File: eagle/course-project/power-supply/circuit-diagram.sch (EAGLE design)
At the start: 10 parts, among them IC1 7805T

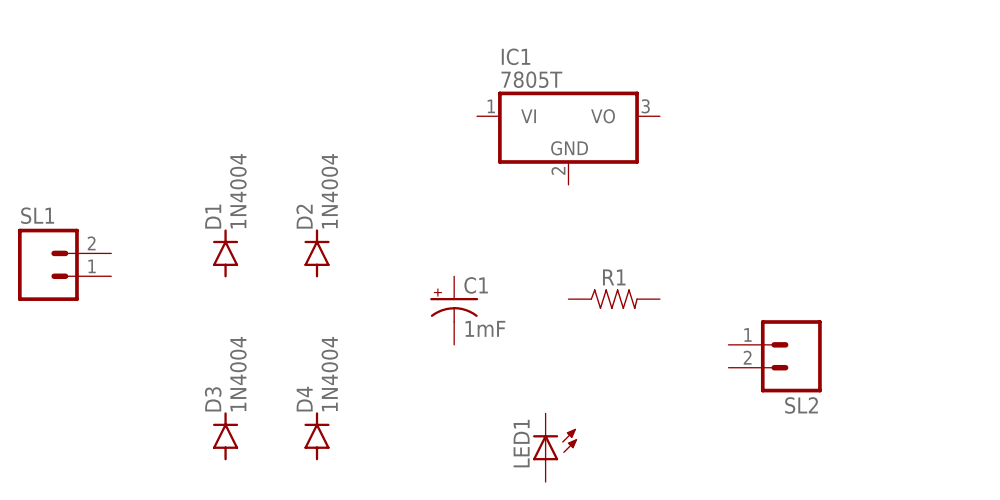
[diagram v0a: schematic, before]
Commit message: adding eagle files for practice
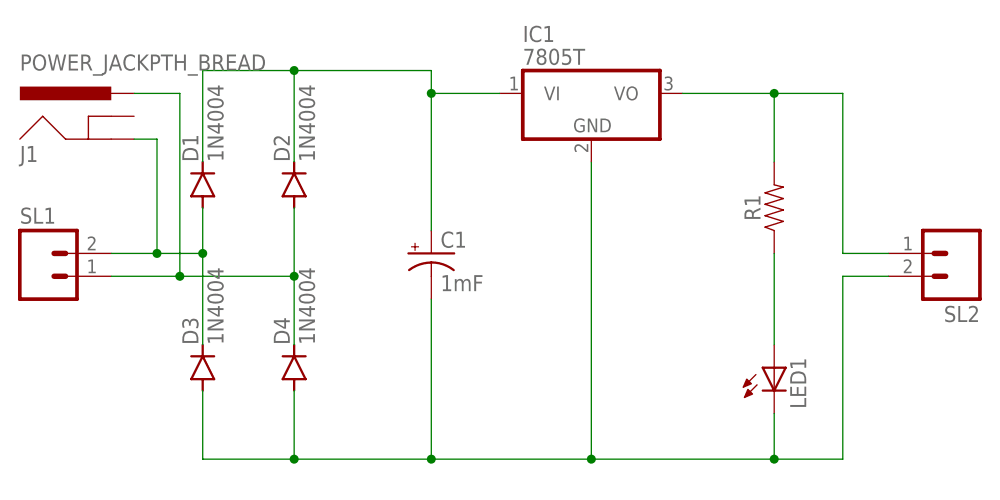
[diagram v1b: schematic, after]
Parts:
- added J1: POWER_JACKPTH_BREAD, SparkFun-Connectors:POWER_JACKPTH_BREAD
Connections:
- new net N$1: D1.A, D3.C, J1.GND, SL1.2
- new net N$2: C1.+, D1.C, D2.C, IC1.VI
- new net N$3: D2.A, D4.C, J1.PWR, SL1.1
- new net N$4: C1.-, D3.A, D4.A, IC1.GND, LED1.C, SL2.2
- new net N$5: IC1.VO, R1.2, SL2.1
- new net N$6: LED1.A, R1.1
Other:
- moved on the sheet: C1, D1, D2, D3, D4, IC1, LED1, R1, SL2
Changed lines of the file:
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@@
 <part name="LED1" library="adafruit" deviceset="LED" device="5MM"/>
 <part name="FRAME1" library="frames" library_urn="urn:adsk.eagle:library:229" deviceset="FRAME_A_L" device=""/>
+<part name="J1" library="SparkFun-Connectors" library_urn="urn:adsk.eagle:library:513" deviceset="POWER_JACK" device="PTH_BREAD" package3d_urn="urn:adsk.eagle:package:38228/1"/>
 </parts>
 <sheets>
@@
 <attribute name="NAME" x="35.56" y="74.422" size="1.778" layer="95"/>
 </instance>
-<instance part="SL2" gate="G$1" x="121.92" y="60.96" smashed="yes" rot="R180">
-<attribute name="VALUE" x="124.46" y="66.04" size="1.778" layer="96" rot="R180"/>
-<attribute name="NAME" x="124.46" y="55.118" size="1.778" layer="95" rot="R180"/>
+<instance part="SL2" gate="G$1" x="139.7" y="71.12" smashed="yes" rot="R180">
+<attribute name="VALUE" x="142.24" y="76.2" size="1.778" layer="96" rot="R180"/>
+<attribute name="NAME" x="142.24" y="65.278" size="1.778" layer="95" rot="R180"/>
 </instance>
-<instance part="D1" gate="1" x="58.42" y="71.12" smashed="yes" rot="R90">
-<attribute name="NAME" x="57.9374" y="73.66" size="1.778" layer="95" rot="R90"/>
-<attribute name="VALUE" x="60.7314" y="73.66" size="1.778" layer="96" rot="R90"/>
+<instance part="D1" gate="1" x="55.88" y="78.74" smashed="yes" rot="R90">
+<attribute name="NAME" x="55.3974" y="81.28" size="1.778" layer="95" rot="R90"/>
+<attribute name="VALUE" x="58.1914" y="81.28" size="1.778" layer="96" rot="R90"/>
 </instance>
-<instance part="D2" gate="1" x="68.58" y="71.12" smashed="yes" rot="R90">
-<attribute name="NAME" x="68.0974" y="73.66" size="1.778" layer="95" rot="R90"/>
-<attribute name="VALUE" x="70.8914" y="73.66" size="1.778" layer="96" rot="R90"/>
+<instance part="D2" gate="1" x="66.04" y="78.74" smashed="yes" rot="R90">
+<attribute name="NAME" x="65.5574" y="81.28" size="1.778" layer="95" rot="R90"/>
+<attribute name="VALUE" x="68.3514" y="81.28" size="1.778" layer="96" rot="R90"/>
 </instance>
-<instance part="D3" gate="1" x="58.42" y="50.8" smashed="yes" rot="R90">
-<attribute name="NAME" x="57.9374" y="53.34" size="1.778" layer="95" rot="R90"/>
-<attribute name="VALUE" x="60.7314" y="53.34" size="1.778" layer="96" rot="R90"/>
+<instance part="D3" gate="1" x="55.88" y="58.42" smashed="yes" rot="R90">
+<attribute name="NAME" x="55.3974" y="60.96" size="1.778" layer="95" rot="R90"/>
+<attribute name="VALUE" x="58.1914" y="60.96" size="1.778" layer="96" rot="R90"/>
 </instance>
-<instance part="D4" gate="1" x="68.58" y="50.8" smashed="yes" rot="R90">
-<attribute name="NAME" x="68.0974" y="53.34" size="1.778" layer="95" rot="R90"/>
-<attribute name="VALUE" x="70.8914" y="53.34" size="1.778" layer="96" rot="R90"/>
+<instance part="D4" gate="1" x="66.04" y="58.42" smashed="yes" rot="R90">
+<attribute name="NAME" x="65.5574" y="60.96" size="1.778" layer="95" rot="R90"/>
+<attribute name="VALUE" x="68.3514" y="60.96" size="1.778" layer="96" rot="R90"/>
 </instance>
-<instance part="C1" gate="G$1" x="83.82" y="66.04" smashed="yes">
-<attribute name="NAME" x="84.836" y="66.675" size="1.778" layer="95" font="vector"/>
-<attribute name="VALUE" x="84.836" y="61.849" size="1.778" layer="96" font="vector"/>
+<instance part="C1" gate="G$1" x="81.28" y="71.12" smashed="yes">
+<attribute name="NAME" x="82.296" y="71.755" size="1.778" layer="95" font="vector"/>
+<attribute name="VALUE" x="82.296" y="66.929" size="1.778" layer="96" font="vector"/>
 </instance>
-<instance part="IC1" gate="A1" x="96.52" y="86.36" smashed="yes">
-<attribute name="NAME" x="88.9" y="92.075" size="1.778" layer="95"/>
-<attribute name="VALUE" x="88.9" y="89.535" size="1.778" layer="96"/>
+<instance part="IC1" gate="A1" x="99.06" y="88.9" smashed="yes">
+<attribute name="NAME" x="91.44" y="94.615" size="1.778" layer="95"/>
+<attribute name="VALUE" x="91.44" y="92.075" size="1.778" layer="96"/>
 </instance>
-<instance part="R1" gate="G$1" x="101.6" y="66.04" smashed="yes">
-<attribute name="NAME" x="101.6" y="67.564" size="1.778" layer="95" font="vector" align="bottom-center"/>
-<attribute name="VALUE" x="101.6" y="64.516" size="1.778" layer="96" font="vector" align="top-center"/>
+<instance part="R1" gate="G$1" x="119.38" y="76.2" smashed="yes" rot="R90">
+<attribute name="NAME" x="117.856" y="76.2" size="1.778" layer="95" font="vector" rot="R90" align="bottom-center"/>
+<attribute name="VALUE" x="120.904" y="76.2" size="1.778" layer="96" font="vector" rot="R90" align="top-center"/>
 </instance>
-<instance part="LED1" gate="G$1" x="93.98" y="48.26" smashed="yes" rot="R180">
-<attribute name="NAME" x="90.424" y="52.832" size="1.778" layer="95" rot="R270"/>
-<attribute name="VALUE" x="88.265" y="52.832" size="1.778" layer="96" rot="R270"/>
+<instance part="LED1" gate="G$1" x="119.38" y="58.42" smashed="yes">
+<attribute name="NAME" x="122.936" y="53.848" size="1.778" layer="95" rot="R90"/>
+<attribute name="VALUE" x="125.095" y="53.848" size="1.778" layer="96" rot="R90"/>
 </instance>
 <instance part="FRAME1" gate="G$1" x="27.94" y="35.56" smashed="yes"/>
@@
 <attribute name="DRAWING_NAME" x="218.44" y="54.61" size="2.54" layer="94"/>
 </instance>
+<instance part="J1" gate="G$1" x="45.72" y="81.28" smashed="yes">
+<attribute name="VALUE" x="35.56" y="91.44" size="1.778" layer="96" font="vector"/>
+<attribute name="NAME" x="35.56" y="81.28" size="1.778" layer="95" font="vector"/>
+</instance>
 </instances>
 <busses>
 </busses>
 <nets>
+<net name="N$1" class="0">
+<segment>
+<pinref part="SL1" gate="G$1" pin="2"/>
+<wire x1="45.72" y1="71.12" x2="50.8" y2="71.12" width="0.1524" layer="91"/>
+<pinref part="D1" gate="1" pin="A"/>
+<wire x1="50.8" y1="71.12" x2="55.88" y2="71.12" width="0.1524" layer="91"/>
+<wire x1="55.88" y1="71.12" x2="55.88" y2="76.2" width="0.1524" layer="91"/>
+<pinref part="D3" gate="1" pin="C"/>
+<wire x1="55.88" y1="60.96" x2="55.88" y2="71.12" width="0.1524" layer="91"/>
+<junction x="55.88" y="71.12"/>
+<pinref part="J1" gate="G$1" pin="GND"/>
+<wire x1="48.26" y1="83.82" x2="50.8" y2="83.82" width="0.1524" layer="91"/>
+<wire x1="50.8" y1="83.82" x2="50.8" y2="71.12" width="0.1524" layer="91"/>
+<junction x="50.8" y="71.12"/>
+</segment>
+</net>
+<net name="N$2" class="0">
+<segment>
+<pinref part="D1" gate="1" pin="C"/>
+<wire x1="55.88" y1="81.28" x2="55.88" y2="91.44" width="0.1524" layer="91"/>
+<wire x1="55.88" y1="91.44" x2="66.04" y2="91.44" width="0.1524" layer="91"/>
+<pinref part="D2" gate="1" pin="C"/>
+<wire x1="66.04" y1="91.44" x2="66.04" y2="81.28" width="0.1524" layer="91"/>
+<wire x1="66.04" y1="91.44" x2="81.28" y2="91.44" width="0.1524" layer="91"/>
+<junction x="66.04" y="91.44"/>
+<pinref part="C1" gate="G$1" pin="+"/>
+<wire x1="81.28" y1="91.44" x2="81.28" y2="88.9" width="0.1524" layer="91"/>
+<pinref part="IC1" gate="A1" pin="VI"/>
+<wire x1="81.28" y1="88.9" x2="81.28" y2="73.66" width="0.1524" layer="91"/>
+<wire x1="88.9" y1="88.9" x2="81.28" y2="88.9" width="0.1524" layer="91"/>
+<junction x="81.28" y="88.9"/>
+</segment>
+</net>
+<net name="N$3" class="0">
+<segment>
+<pinref part="D2" gate="1" pin="A"/>
+<pinref part="D4" gate="1" pin="C"/>
+<wire x1="66.04" y1="76.2" x2="66.04" y2="68.58" width="0.1524" layer="91"/>
+<pinref part="SL1" gate="G$1" pin="1"/>
+<wire x1="66.04" y1="68.58" x2="66.04" y2="60.96" width="0.1524" layer="91"/>
+<junction x="66.04" y="68.58"/>
+<wire x1="45.72" y1="68.58" x2="53.34" y2="68.58" width="0.1524" layer="91"/>
+<pinref part="J1" gate="G$1" pin="PWR"/>
+<wire x1="53.34" y1="68.58" x2="66.04" y2="68.58" width="0.1524" layer="91"/>
+<wire x1="48.26" y1="88.9" x2="53.34" y2="88.9" width="0.1524" layer="91"/>
+<wire x1="53.34" y1="88.9" x2="53.34" y2="68.58" width="0.1524" layer="91"/>
+<junction x="53.34" y="68.58"/>
+</segment>
+</net>
+<net name="N$4" class="0">
+<segment>
+<pinref part="D3" gate="1" pin="A"/>
+<wire x1="55.88" y1="55.88" x2="55.88" y2="48.26" width="0.1524" layer="91"/>
+<wire x1="55.88" y1="48.26" x2="66.04" y2="48.26" width="0.1524" layer="91"/>
+<pinref part="D4" gate="1" pin="A"/>
+<wire x1="66.04" y1="48.26" x2="66.04" y2="55.88" width="0.1524" layer="91"/>
+<pinref part="C1" gate="G$1" pin="-"/>
+<wire x1="81.28" y1="66.04" x2="81.28" y2="48.26" width="0.1524" layer="91"/>
+<wire x1="81.28" y1="48.26" x2="66.04" y2="48.26" width="0.1524" layer="91"/>
+<junction x="66.04" y="48.26"/>
+<pinref part="IC1" gate="A1" pin="GND"/>
+<wire x1="99.06" y1="81.28" x2="99.06" y2="48.26" width="0.1524" layer="91"/>
+<wire x1="99.06" y1="48.26" x2="81.28" y2="48.26" width="0.1524" layer="91"/>
+<junction x="81.28" y="48.26"/>
+<wire x1="99.06" y1="48.26" x2="119.38" y2="48.26" width="0.1524" layer="91"/>
+<junction x="99.06" y="48.26"/>
+<pinref part="LED1" gate="G$1" pin="C"/>
+<wire x1="119.38" y1="48.26" x2="119.38" y2="53.34" width="0.1524" layer="91"/>
+<wire x1="127" y1="68.58" x2="127" y2="48.26" width="0.1524" layer="91"/>
+<wire x1="127" y1="48.26" x2="119.38" y2="48.26" width="0.1524" layer="91"/>
+<junction x="119.38" y="48.26"/>
+<pinref part="SL2" gate="G$1" pin="2"/>
+<wire x1="132.08" y1="68.58" x2="127" y2="68.58" width="0.1524" layer="91"/>
+</segment>
+</net>
+<net name="N$5" class="0">
+<segment>
+<pinref part="SL2" gate="G$1" pin="1"/>
+<wire x1="132.08" y1="71.12" x2="127" y2="71.12" width="0.1524" layer="91"/>
+<wire x1="127" y1="71.12" x2="127" y2="88.9" width="0.1524" layer="91"/>
+<pinref part="R1" gate="G$1" pin="2"/>
+<wire x1="119.38" y1="88.9" x2="119.38" y2="81.28" width="0.1524" layer="91"/>
+<pinref part="IC1" gate="A1" pin="VO"/>
+<wire x1="109.22" y1="88.9" x2="119.38" y2="88.9" width="0.1524" layer="91"/>
+<wire x1="127" y1="88.9" x2="119.38" y2="88.9" width="0.1524" layer="91"/>
+<junction x="119.38" y="88.9"/>
+</segment>
+</net>
+<net name="N$6" class="0">
+<segment>
+<pinref part="R1" gate="G$1" pin="1"/>
+<pinref part="LED1" gate="G$1" pin="A"/>
+<wire x1="119.38" y1="71.12" x2="119.38" y2="60.96" width="0.1524" layer="91"/>
+</segment>
+</net>
 </nets>
 </sheet>
